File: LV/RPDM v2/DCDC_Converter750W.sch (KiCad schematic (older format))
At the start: 16 parts

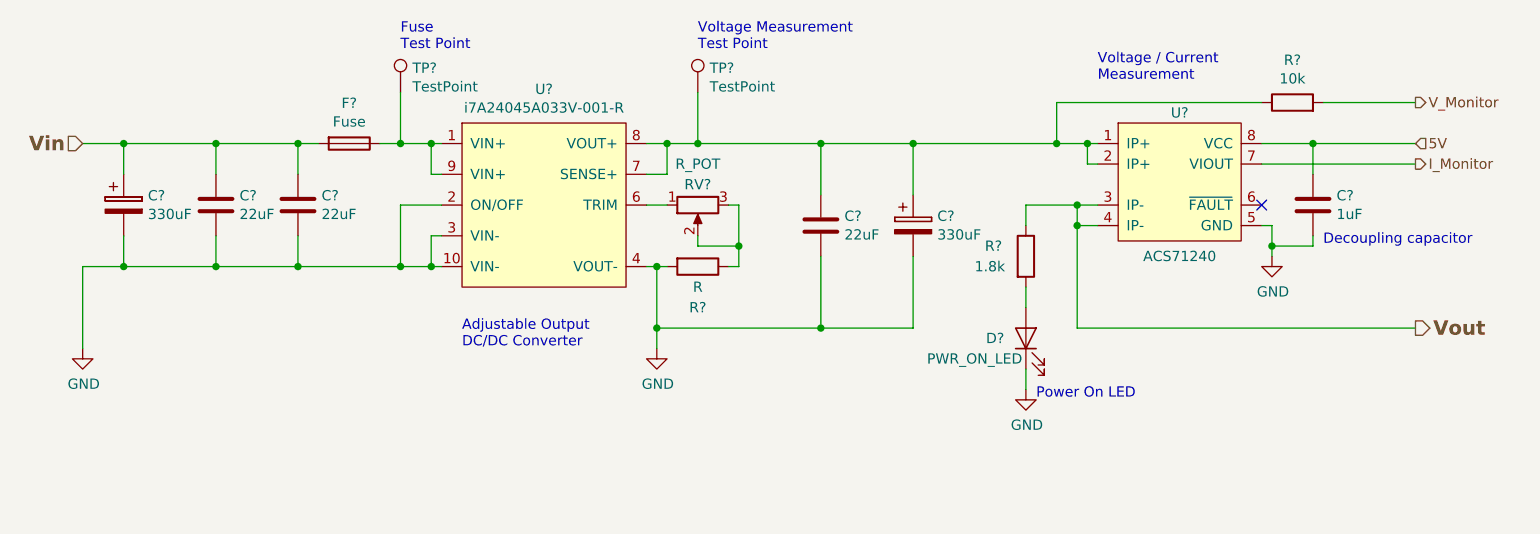
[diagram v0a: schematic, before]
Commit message: RPDM update
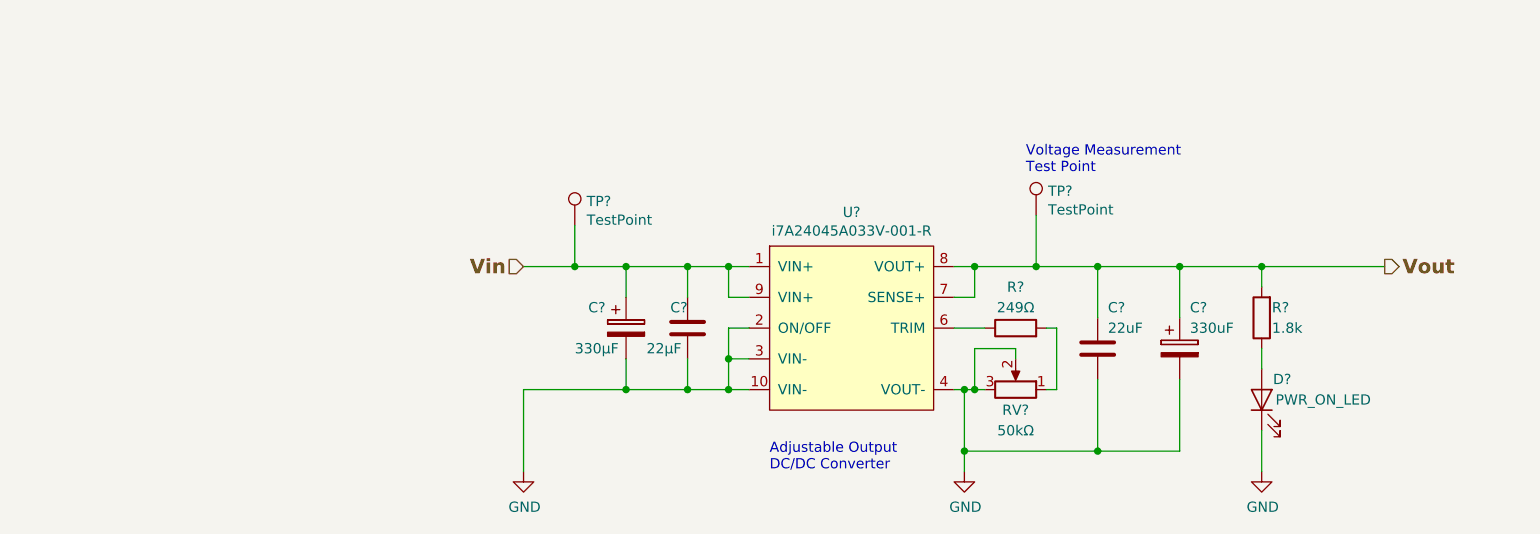
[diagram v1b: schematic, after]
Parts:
- removed C?: 22uF, symbol Device:C
- removed C?: 1uF, symbol Device:C
- removed F?: Fuse, symbol Device:Fuse
- removed R?: 10k, symbol Device:R
- removed U?: ACS71240, symbol sensor_current_allegro:ACS71240
- C?: value 330uF -> 330µF
- C?: value 22uF -> 22µF
- R?: value R -> 249Ω
- RV?: value R_POT -> 50kΩ
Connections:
- net GND: now also RV?.2, RV?.3; no longer R?.2
- net Vin: now also TP?.1, U?.1 (VIN+), U?.9 (VIN+)
- net Vout: now also C?.1, C?.1, R?.2, TP?.1, U?.7 (SENSE+), U?.8 (VOUT+); no longer R?.1
- net at RV?.1: now also R?.2; no longer U?.6 (TRIM)
- net at D?.2 (A): now also R?.1; no longer R?.2
- new net: R?.1, U?.6 (TRIM)
- no-connect marks 1 -> 0
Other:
- note removed: "Decoupling capacitor"
- note removed: "Fuse\nTest Point"
- note removed: "Power On LED"
- note removed: "Voltage / Current\nMeasurement"
- moved on the sheet: C?, D?, R?, RV?, TP?, U?
